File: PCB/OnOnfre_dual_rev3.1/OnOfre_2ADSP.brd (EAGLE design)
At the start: 53 x 55 mm, 23 parts, among them J1 4p, J6 8p, J7 8p, K1 OMRON-G3MB-202P-SSR2, K2 OMRON-G3MB-202P-SSR2, Q1 S8050, Q2 S8050, U1 LM1117, U2 esp12

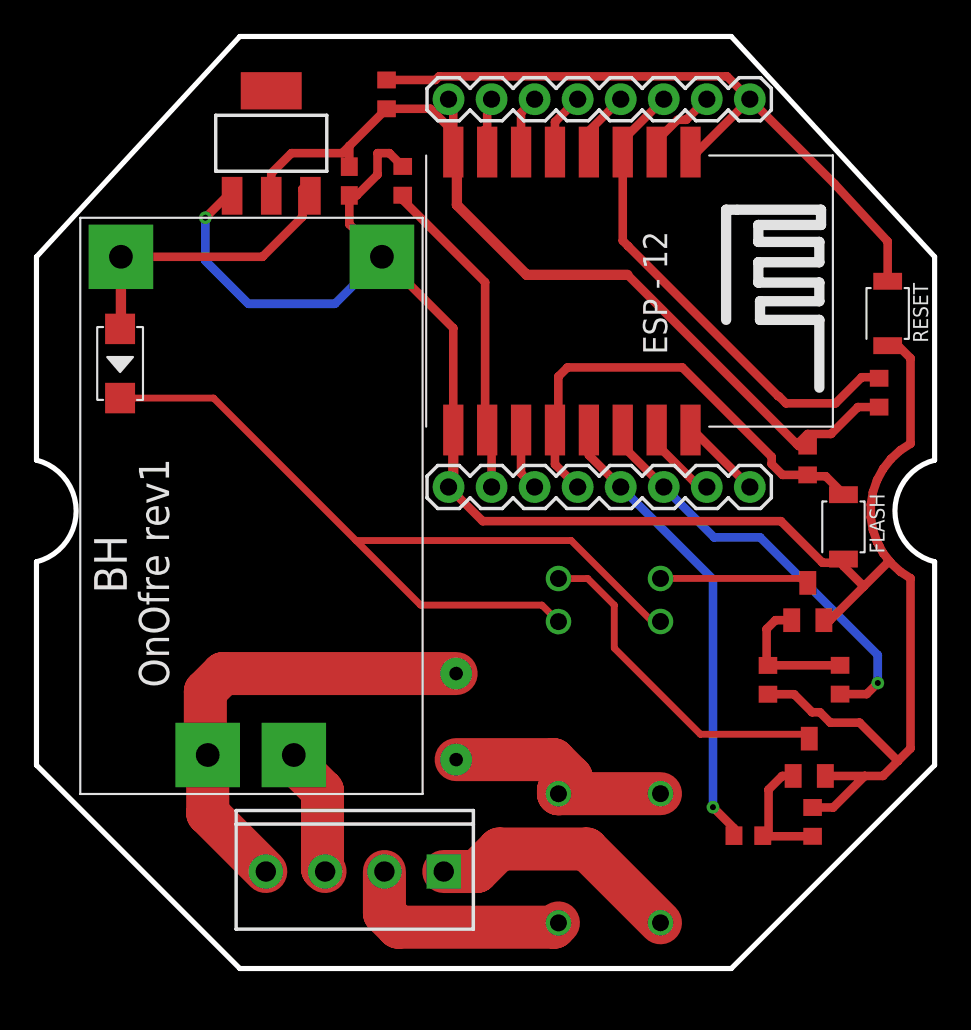
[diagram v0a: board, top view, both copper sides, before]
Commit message: Rev3.1 dual
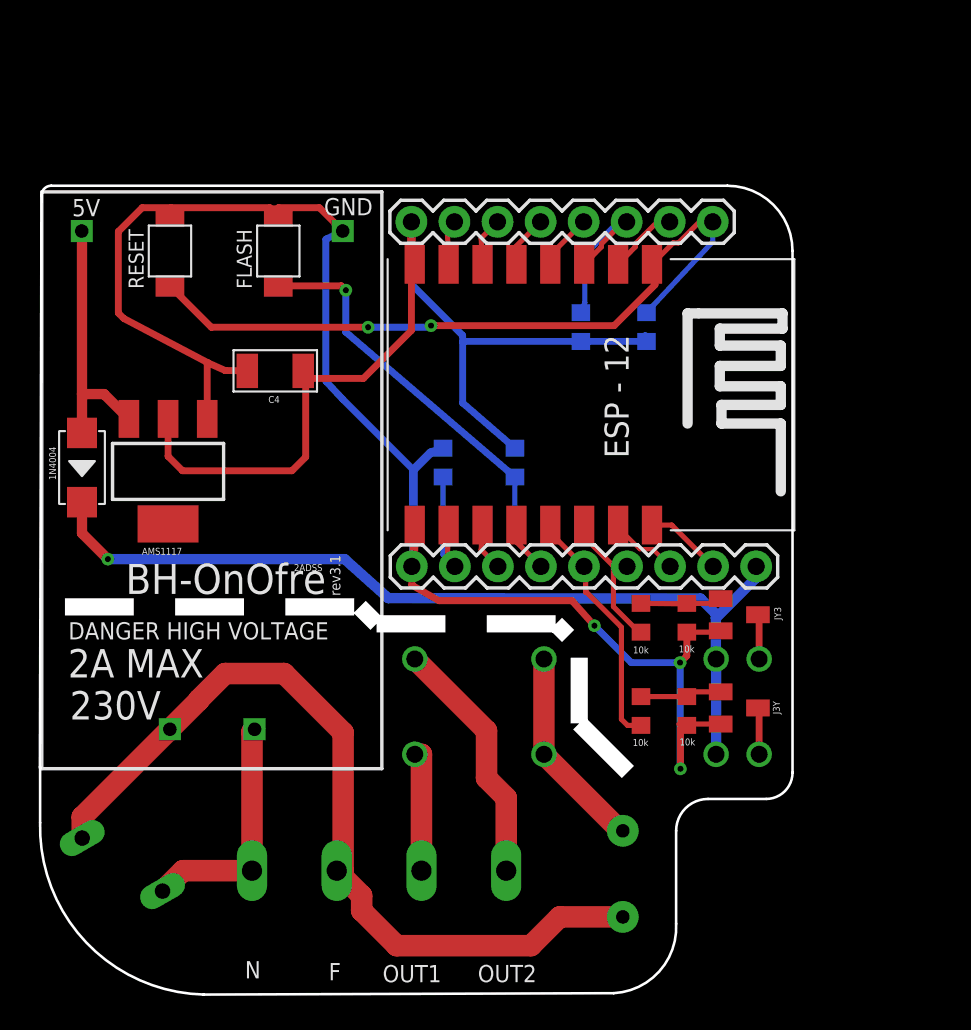
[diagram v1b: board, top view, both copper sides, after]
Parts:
- removed J1: 4p, SparkFun-Connectors:SCREWTERMINAL-3.5MM-4
- removed Q1, Q2: S8050, semicon-smd-ipc:SOT23
- removed U1: LM1117, SparkFun-IC-Power:SOT223
- added AMS1117: LM1117, SparkFun-IC-Power:SOT223
- added J3Y, JY3: S8050, semicon-smd-ipc:SOT23
- added R5: VARISTORS07K230, varistor:S07K230
- added X1: (no value), con-wago-500:W237-4
- C4: value 100nF -> 100NF; device SparkFun-Capacitors:0603 -> Seeed-Capacitor:C1206
- FLASH, RESET: device Seeed-Switch:SW2-2.6-3.0X2.5X1.2+0.4MM -> switches:B3U-1000P
- J6: device SparkFun-Connectors:1X08 -> SparkFun-Connectors:1X09
- U$2: value HLK-PM03 -> HKLPM01; device PowerSocket:HLK-PM03 -> HKLPM01:HKLPM01
- moved RESET 42.5 mm to (8.07, 42.5), turned to 90 degrees
- moved FLASH 37.1 mm to (14.5, 42.5), turned to 90 degrees
- moved R10 20.6 mm to (36.2, 38.0), flipped to the bottom
- moved R9 18.0 mm to (32.3, 38.0), flipped to the bottom
- moved R8 17.3 mm to (28.4, 30.0), flipped to the bottom
- moved U$2 16.9 mm to (10.6, 29.0), flipped to the bottom
- moved R11 16.8 mm to (24.2, 30.0), flipped to the bottom
- moved F1 13.5 mm to (34.8, 5.73), turned to 90 degrees
- moved R1 12.3 mm to (35.9, 20.8)
- moved C4 12.0 mm to (14.3, 35.4), turned to 180 degrees
- moved R3 9.89 mm to (38.6, 15.3), turned to 90 degrees
- moved R4 9.71 mm to (35.9, 15.3), turned to 90 degrees
- moved J7 7.56 mm to (22.3, 44.2)
- moved D3 6.54 mm to (2.88, 29.7)
- moved U2 6.53 mm to (30.7, 33.9)
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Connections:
- removed net FASE: J1.3, U$2.AC2
- removed net N$2: D3.2, K1.3, K2.3
- new net FASE_IN: R5.1, U$2.P$1, X1.1
- new net VCC_D: D3.2, J6.9, K1.3, K2.3
- net 3V3: now also AMS1117.2; no longer U1.2
- net GND: now also AMS1117.1, J3Y.2, JY3.2, U$2.P$3; no longer Q1.2, Q2.2, U$2.-VO, U1.1
- net N$1: now also J3Y.3; no longer Q1.3
- net N$13: now also JY3.1; no longer Q2.1
- net N$7: now also J3Y.1; no longer Q1.1
- net N$9: now also JY3.3; no longer Q2.3
- net NEUTRAL_IN: now also R5.2, U$2.P$2, X1.2; no longer J1.4, U$2.AC1
- net NEUTRAL_ONE_OUT: now also X1.3; no longer J1.2
- net NEUTRAL_TWO_OUT: now also X1.4; no longer J1.1
- net VCC: now also AMS1117.3, U$2.P$4; no longer U$2.+VO, U1.3
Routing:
- net VCC_D: track 0.00 -> 53.4 mm, vias 0 -> 1
- net N$2: track 51.3 -> 0.00 mm
- net GND: track 120.8 -> 95.4 mm, vias 1 -> 3
- net NEUTRAL_IN: track 27.3 -> 50.1 mm
- net CH_PD: track 29.4 -> 10.4 mm
- net N$1: track 20.2 -> 2.76 mm
- net GPIO04: track 25.2 -> 8.64 mm, vias 1 -> 0
- net FASE_IN: track 0.00 -> 14.2 mm
- net GPIO05: track 27.5 -> 14.6 mm, vias 1 -> 0
- net GPIO15: track 19.6 -> 8.19 mm
- net FASE: track 7.64 -> 0.00 mm
- net N$9: track 8.80 -> 2.64 mm
- net NEUTRAL_ONE_OUT: track 13.2 -> 7.26 mm
- net 3V3: track 55.6 -> 60.2 mm
- net N$13: track 8.24 -> 4.93 mm
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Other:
- board size 53 x 55 mm -> 44.4 x 47.7 mm
- board text added: "00"
- board text added: "02"
- board text added: "04"
- board text added: "05"
- board text added: "12"
- board text added: "13"
- board text added: "14"
- board text added: "15"
- board text added: "16"
- board text added: "230V"
- board text added: "2A MAX"
- board text added: "2ADSS"
- board text added: "3V3"
- board text added: "5V"
- board text added: "ADC"
- board text added: "BH-OnOfre"
- board text added: "DANGER HIGH VOLTAGE"
- board text added: "EN"
- board text added: "F"
- board text added: "GND"
- board text added: "HLK-PM01"
- board text added: "N"
- board text added: "OUT1"
- board text added: "OUT2"
- board text added: "RST"
- board text added: "RX"
- board text added: "TX"
- board text added: "rev3.1"
- board text removed: "BH"
- board text removed: "OnOfre rev1"
